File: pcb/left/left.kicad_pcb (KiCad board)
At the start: 2 copper layers, 35.6 x 58.4 mm, 21 parts

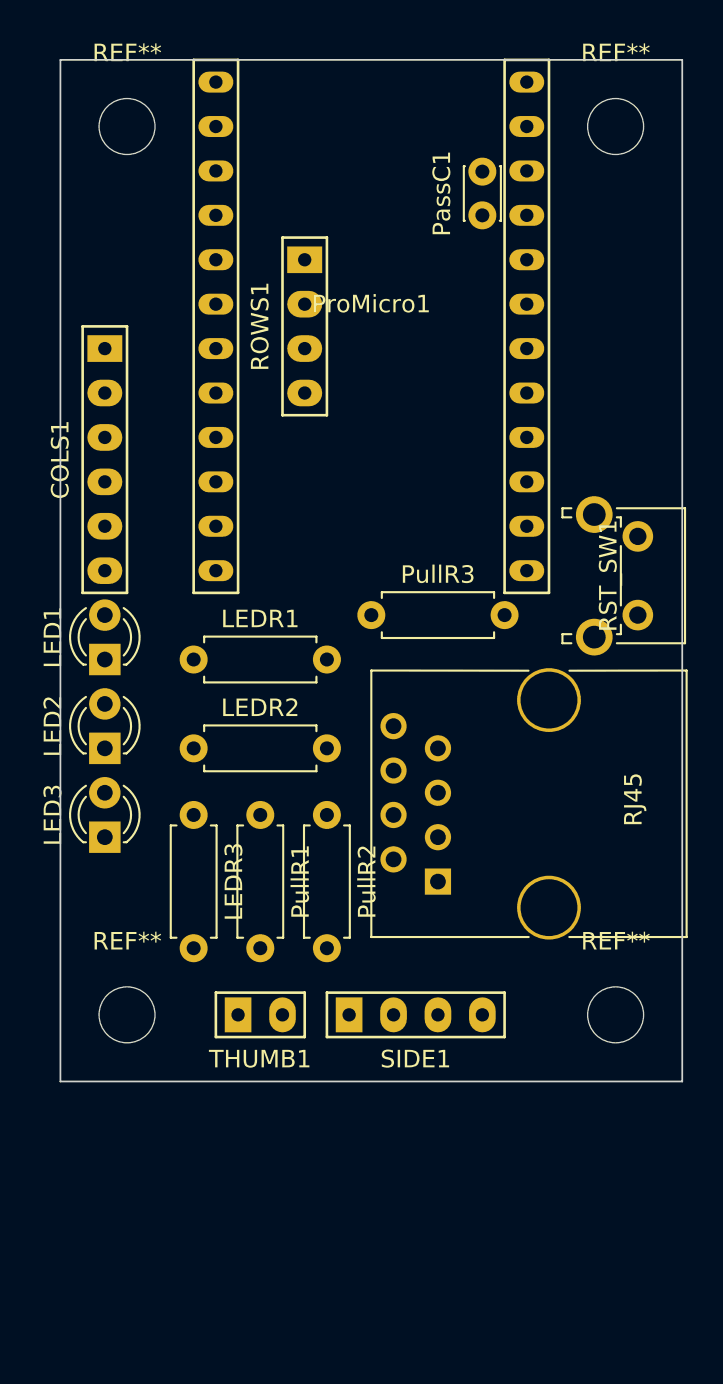
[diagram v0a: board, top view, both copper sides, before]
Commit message: improve basic design
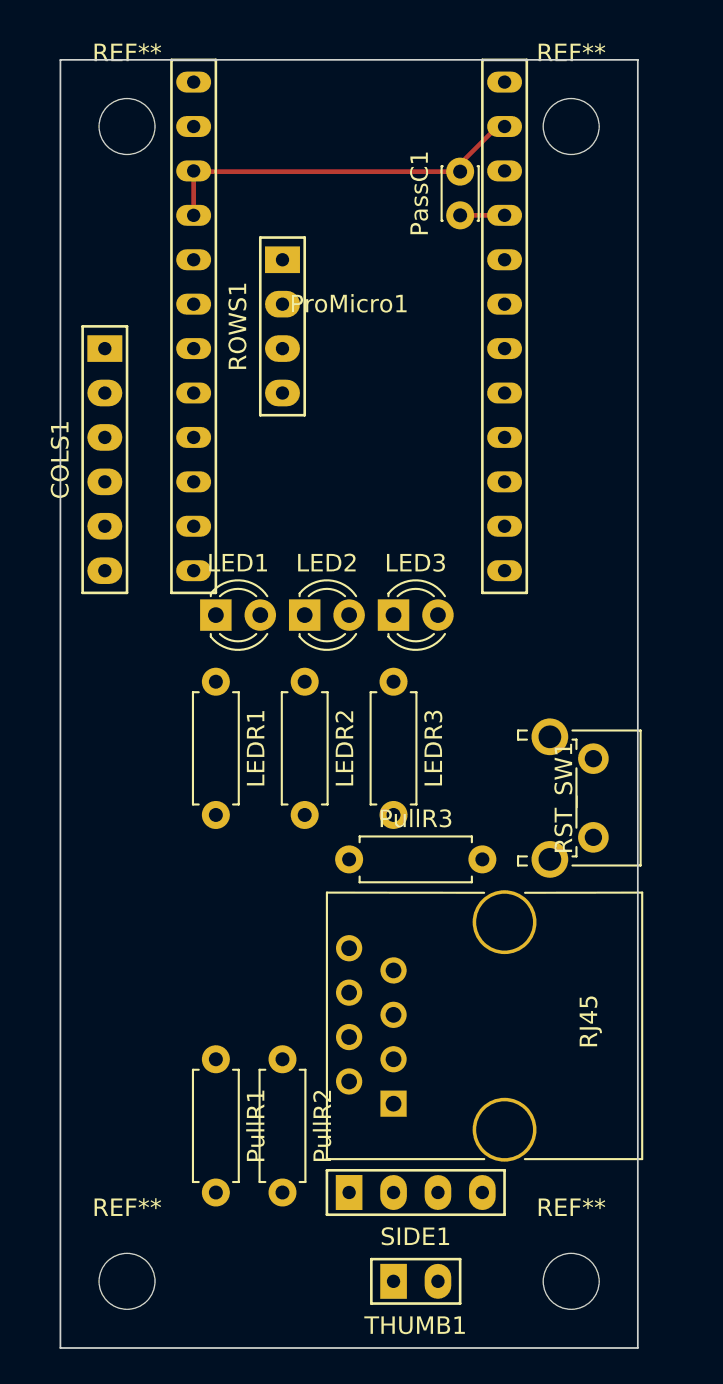
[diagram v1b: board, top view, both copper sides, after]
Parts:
- moved LED3 20.8 mm to (15.2, 27.9), turned to 0 degrees
- moved THUMB1 17.6 mm to (16.5, 66.0)
- moved REF** 15.5 mm to (25.4, 66.0)
- moved REF** 15.2 mm to (0.00, 66.0)
- moved PullR1 14.2 mm to (5.08, 53.3)
- moved PullR2 14.2 mm to (8.89, 53.3)
- moved PullR3 14.0 mm to (12.7, 41.9)
- moved LED2 13.7 mm to (10.2, 27.9), turned to 0 degrees
- moved LEDR3 13.7 mm to (15.2, 31.8)
- moved RST_SW1 13.0 mm to (26.7, 36.1)
- moved RJ45 13.0 mm to (15.2, 55.9)
- moved SIDE1 10.2 mm to (16.5, 61.0)
- moved LEDR2 7.41 mm to (10.2, 31.8), turned to 270 degrees
- moved LED1 6.84 mm to (5.08, 27.9), turned to 0 degrees
- moved REF** 2.54 mm to (25.4, 0.00)
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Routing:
- net GND: track 0.00 -> 21.7 mm
- net +5V: track 0.00 -> 2.54 mm
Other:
- board size 35.6 x 58.4 mm -> 33 x 73.7 mm
